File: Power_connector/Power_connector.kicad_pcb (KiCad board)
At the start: 2 copper layers, 184.8 x 60.3 mm, 54 parts, among them J1 XT60_F, J10 XT60_F, J11 XT60_F, J12 XT60_F, J13 XT60_F, J14 XT60_F, J2 XT60_Male, J3 XT60_F, J4 XT60_F, J5 Screw_Terminal_01x02, J6 XT60_F, J7 XT60_F, J8 XT60_F, J9 XT60_F, Q1 IRFS7530, Q2 IRFS7530, Q3 IRFS7530, Q4 IRFS7530

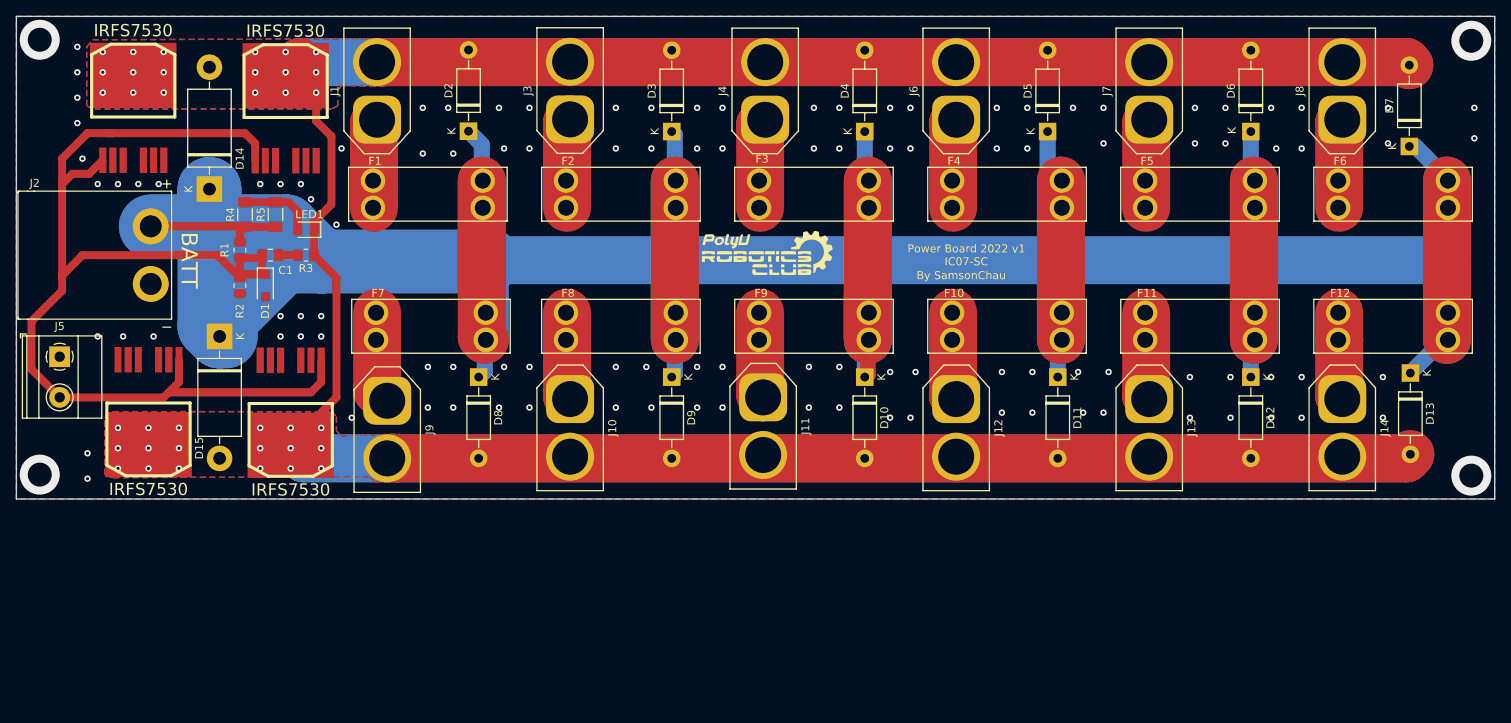
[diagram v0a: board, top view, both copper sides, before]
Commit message: powerboard mod
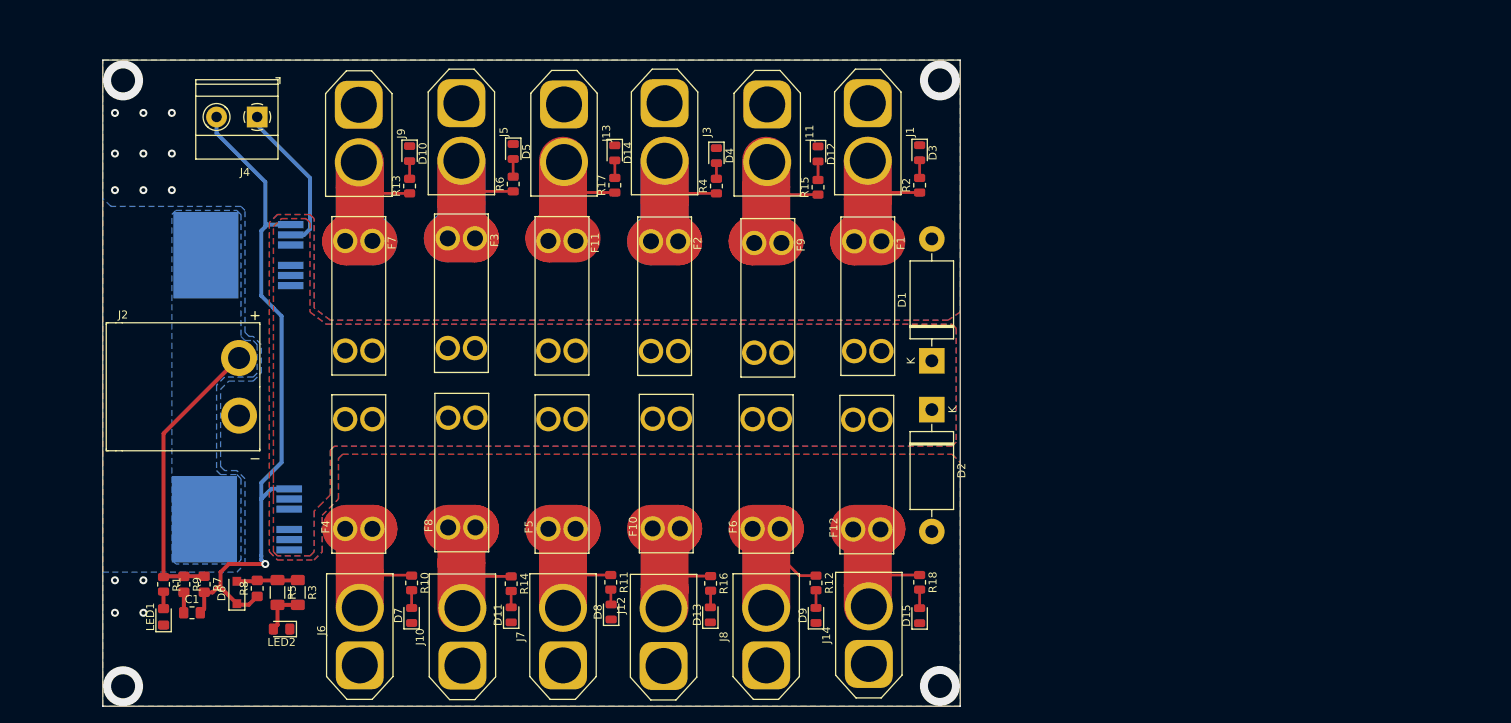
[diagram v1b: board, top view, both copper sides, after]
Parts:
- removed G*** (x2): LOGO, PolyuRobotics:Club_logo
- removed Q3, Q4: IRFS7530, sparkparts:D2PAK-7-GDS
- added LED2: power, LED_SMD:LED_0805_2012Metric_Pad1.15x1.40mm_HandSolder, F.Cu at (98.6, 125.5)
- added R10: 10M, Resistor_SMD:R_0805_2012Metric, F.Cu at (114.8, 119.7)
- added R11: 10M, Resistor_SMD:R_0805_2012Metric, F.Cu at (139.7, 119.6)
- added R12: 10M, Resistor_SMD:R_0805_2012Metric, F.Cu at (165.4, 119.7)
- added R13: 10M, Resistor_SMD:R_0805_2012Metric, F.Cu at (114.6, 70.1)
- added R14: 10M, Resistor_SMD:R_0805_2012Metric, F.Cu at (127.3, 119.8)
- added R15: 10M, Resistor_SMD:R_0805_2012Metric, F.Cu at (165.6, 70.3)
- added R16: 10M, Resistor_SMD:R_0805_2012Metric, F.Cu at (152.2, 119.8)
- added R17: 10M, Resistor_SMD:R_0805_2012Metric, F.Cu at (140.2, 70.0)
- added R18: 10M, Resistor_SMD:R_0805_2012Metric, F.Cu at (178.3, 119.6)
- added R6: 10M, Resistor_SMD:R_0805_2012Metric, F.Cu at (127.5, 69.8)
- added R7: 1.5M, Resistor_SMD:R_0805_2012Metric_Pad1.20x1.40mm_HandSolder, F.Cu at (88.9, 119.9)
- added R8: 400k, Resistor_SMD:R_0805_2012Metric_Pad1.20x1.40mm_HandSolder, F.Cu at (95.5, 120.4)
- added R9: 1K, Resistor_SMD:R_0805_2012Metric_Pad1.20x1.40mm_HandSolder, F.Cu at (86.3, 119.9)
- D1: value Zener -> 1N5408; footprint Diode_SMD:D_SOD-123F -> Diode_THT:D_DO-201AD_P15.24mm_Horizontal
- D10, D11, D12, D13, D3, D4, D5, D7, D8, D9: value 1N4001 -> indicator; footprint Diode_THT:D_DO-41_SOD81_P10.16mm_Horizontal -> LED_SMD:LED_0805_2012Metric
- D14, D15: value 1N5408 -> indicator; footprint Diode_THT:D_DO-201AD_P15.24mm_Horizontal -> LED_SMD:LED_0805_2012Metric
- D2: value 1N4001 -> 1N5408; footprint Diode_THT:D_DO-41_SOD81_P10.16mm_Horizontal -> Diode_THT:D_DO-201AD_P15.24mm_Horizontal
- D6: value 1N4001 -> Zener; footprint Diode_THT:D_DO-41_SOD81_P10.16mm_Horizontal -> Diode_SMD:D_SOD-123F
- J4: value XT60_F -> E_Stop; footprint Connector_AMASS:AMASS_XT60-F_1x02_P7.20mm_Vertical -> TerminalBlock_Phoenix:TerminalBlock_Phoenix_MKDS-1,5-2-5.08_1x02_P5.08mm_Horizontal
- J5: value Screw_Terminal_01x02 -> XT60_F; footprint TerminalBlock_Phoenix:TerminalBlock_Phoenix_MKDS-1,5-2-5.08_1x02_P5.08mm_Horizontal -> Connector_AMASS:AMASS_XT60-F_1x02_P7.20mm_Vertical
- LED1: value power -> BATT
- Q1, Q2: moved to B.Cu
- R1: value 1.5M -> 10M; footprint Resistor_SMD:R_0805_2012Metric_Pad1.20x1.40mm_HandSolder -> Resistor_SMD:R_0805_2012Metric
- R2: value 400k -> 10M; footprint Resistor_SMD:R_0805_2012Metric_Pad1.20x1.40mm_HandSolder -> Resistor_SMD:R_0805_2012Metric
- R3: value 1K -> 16.5K; footprint Resistor_SMD:R_0805_2012Metric_Pad1.20x1.40mm_HandSolder -> Resistor_SMD:R_1206_3216Metric_Pad1.30x1.75mm_HandSolder
- R4: value 16.5K -> 10M; footprint Resistor_SMD:R_1206_3216Metric_Pad1.30x1.75mm_HandSolder -> Resistor_SMD:R_0805_2012Metric
- moved D6 139.2 mm to (93.0, 120.9)
- moved D7 137.8 mm to (114.8, 123.8)
- moved J6 101.0 mm to (108.3, 130.0)
- moved J7 100.1 mm to (133.7, 130.0)
- moved J8 99.2 mm to (159.1, 130.0)
- moved D15 94.2 mm to (178.3, 123.8), turned to 90 degrees
- moved D13 92.6 mm to (152.1, 123.7), turned to 90 degrees
- moved F4 88.3 mm to (108.2, 106.1), turned to 90 degrees
- moved F5 87.1 mm to (133.6, 106.1), turned to 90 degrees
- moved R2 85.9 mm to (178.3, 70.0), turned to 90 degrees
- moved F6 85.8 mm to (159.1, 106.1), turned to 90 degrees
- moved D1 83.8 mm to (179.8, 91.9), turned to 90 degrees
- moved J13 81.9 mm to (133.9, 59.9)
- moved F11 79.8 mm to (133.6, 83.8), turned to -90 degrees
- moved D11 74.5 mm to (127.3, 123.7), turned to 90 degrees
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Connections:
- D1 pad 1: /SW_NC -> +24V
- D1 pad 2: -BATT -> GND
- D10 pad 1: +24V -> GND
- D10 pad 2: GND -> Net-(D10-Pad2)
- D11 pad 1: +24V -> GND
- D11 pad 2: GND -> Net-(D11-Pad2)
- D12 pad 1: +24V -> unconnected-(D12-Pad1)
- D12 pad 2: GND -> Net-(D12-Pad2)
- D13 pad 1: +24V -> GND
- D13 pad 2: GND -> Net-(D13-Pad2)
- D14 pad 1: +24V -> GND
- D14 pad 2: GND -> Net-(D14-Pad2)
- D15 pad 1: +24V -> GND
- D15 pad 2: GND -> Net-(D15-Pad2)
- D3 pad 1: +24V -> GND
- D3 pad 2: GND -> Net-(D3-Pad2)
- D4 pad 1: +24V -> GND
- D4 pad 2: GND -> Net-(D4-Pad2)
- D5 pad 1: +24V -> unconnected-(D5-Pad1)
- D5 pad 2: GND -> Net-(D5-Pad2)
- D6 pad 1: +24V -> /SW_NC
- D6 pad 2: GND -> +24V
- D7 pad 1: +24V -> GND
- D7 pad 2: GND -> Net-(D7-Pad2)
- D8 pad 1: +24V -> GND
- D8 pad 2: GND -> Net-(D8-Pad2)
- D9 pad 1: +24V -> GND
- D9 pad 2: GND -> Net-(D9-Pad2)
- J1 pad 1: Net-(F1-Pad1) -> GND
- J1 pad 2: GND -> Net-(F1-Pad1)
- J10 pad 1: Net-(F8-Pad1) -> GND
- J10 pad 2: GND -> Net-(F8-Pad1)
- J11 pad 1: Net-(F9-Pad1) -> GND
- J11 pad 2: GND -> Net-(F9-Pad1)
- J12 pad 1: Net-(F10-Pad1) -> GND
- J12 pad 2: GND -> Net-(F10-Pad1)
- J13 pad 1: Net-(F11-Pad1) -> GND
- J13 pad 2: GND -> Net-(F11-Pad1)
- J14 pad 1: Net-(F12-Pad1) -> GND
- J14 pad 2: GND -> Net-(F12-Pad1)
- J2 pad 1: -BATT -> GND
- J2 pad 2: +24V -> +BATT
- J3 pad 1: Net-(F2-Pad1) -> GND
- J3 pad 2: GND -> Net-(F2-Pad1)
- J4 pad 1: Net-(F3-Pad1) -> +24V
- J4 pad 2: GND -> /SW_NC
- J5 pad 1: -BATT -> GND
- J5 pad 2: /SW_NC -> Net-(F3-Pad1)
- J6 pad 1: Net-(F4-Pad1) -> GND
- J6 pad 2: GND -> Net-(F4-Pad1)
- J7 pad 1: Net-(F5-Pad1) -> GND
- J7 pad 2: GND -> Net-(F5-Pad1)
- J8 pad 1: Net-(F6-Pad1) -> GND
- J8 pad 2: GND -> Net-(F6-Pad1)
- J9 pad 1: Net-(F7-Pad1) -> GND
- J9 pad 2: GND -> Net-(F7-Pad1)
- Q1 pad D: GND -> +BATT
- Q1 pad S: -BATT -> +24V
- Q2 pad D: GND -> +BATT
- Q2 pad S: -BATT -> +24V
- R1 pad 1: +24V -> +BATT
- R1 pad 2: /SW_NC -> Net-(LED1-Pad2)
- R2 pad 1: /SW_NC -> Net-(F1-Pad1)
- R2 pad 2: -BATT -> Net-(D3-Pad2)
- R3 pad 1: GND -> +24V
- R3 pad 2: Net-(C1-Pad1) -> Net-(LED2-Pad2)
- R4 pad 1: +24V -> Net-(F2-Pad1)
- R4 pad 2: Net-(LED1-Pad2) -> Net-(D4-Pad2)
- R5 pad 2: Net-(LED1-Pad2) -> Net-(LED2-Pad2)
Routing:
- net +24V: track 621.5 -> 27.1 mm
- net GND: track 585.0 -> 0.00 mm, vias 36 -> 13
- net /SW_NC: track 144.5 -> 87.1 mm, vias 0 -> 1
- net +BATT: track 0.00 -> 36.4 mm
- net Net-(F2-Pad1): track 11.2 -> 31.8 mm
- net Net-(F3-Pad1): track 11.3 -> 31.3 mm
- net Net-(F7-Pad1): track 11.5 -> 31.1 mm
- net Net-(F6-Pad1): track 11.2 -> 21.9 mm
- net Net-(F9-Pad1): track 10.7 -> 21.0 mm
- net Net-(F8-Pad1): track 11.0 -> 20.9 mm
- net Net-(F1-Pad1): track 11.2 -> 21.0 mm
- net Net-(F12-Pad1): track 11.0 -> 20.8 mm
- net Net-(F11-Pad1): track 11.0 -> 20.5 mm
- net Net-(F10-Pad1): track 11.0 -> 20.4 mm
- net Net-(F4-Pad1): track 11.2 -> 20.5 mm
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- added copper zone on B.Cu, net +24V
- added copper zone on F.Cu, net +24V
- added copper zone on B.Cu, net +BATT
- removed copper zone on B.Cu, net -BATT
- removed copper zone on F.Cu, net -BATT
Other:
- board size 184.8 x 60.3 mm -> 107.2 x 80.8 mm
- board text removed: "BATT"
- board text removed: "By SamsonChau"
- board text removed: "Power Board 2022 v1 IC07-SC"
